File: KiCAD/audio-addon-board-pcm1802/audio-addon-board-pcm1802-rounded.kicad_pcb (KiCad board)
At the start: 4 copper layers, 85 x 70 mm, 69 parts, among them J1 RCA, J2 CONN_HOST_1, J3 RCA, J4 RCA, J5 RCA, SW1 SW_DIP_x04, U1 PCM1802DBR, U2 LTC1682IS8-5, U3 SN74LVC1G125DBV

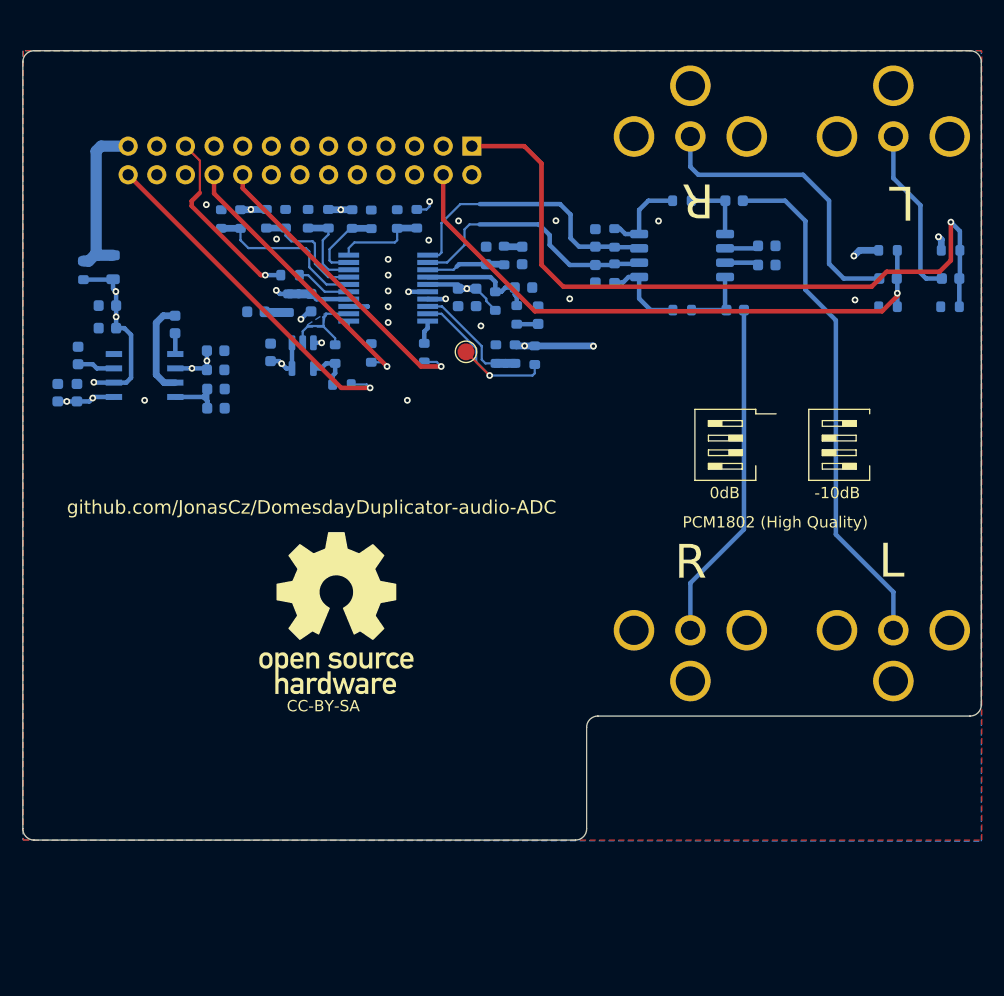
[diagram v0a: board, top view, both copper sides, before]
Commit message: working on layout (2025-10-09 sent to jlc)
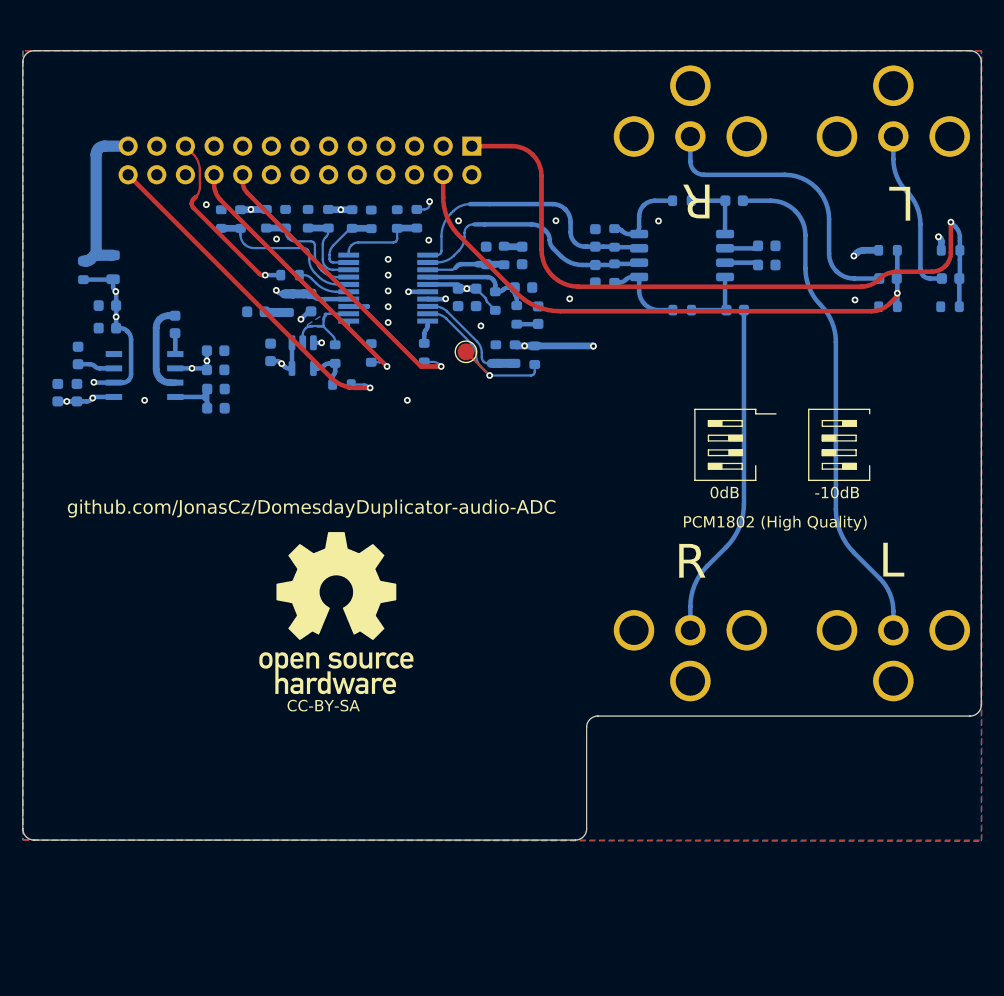
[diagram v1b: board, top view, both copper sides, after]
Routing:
- net +3.3V: track 88.0 -> 86.6 mm
- net /+5V, Analog: track 74.0 -> 72.8 mm
- net Net-(J4-In): track 45.8 -> 44.6 mm
- net Net-(U2-CPO): track 6.17 -> 5.13 mm
- net Net-(J2-Pin_1): track 65.1 -> 64.1 mm
- net Net-(J1-In): track 26.8 -> 26.1 mm
- net GND: track 53.9 -> 53.2 mm
- net Net-(J2-Pin_4): track 53.5 -> 52.8 mm
- net Net-(U1-OSR): track 14.8 -> 14.2 mm
- net VINR: track 23.1 -> 22.5 mm
- net VINL: track 25.0 -> 24.4 mm
- net Net-(J5-In): track 30.4 -> 29.9 mm

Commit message: update board
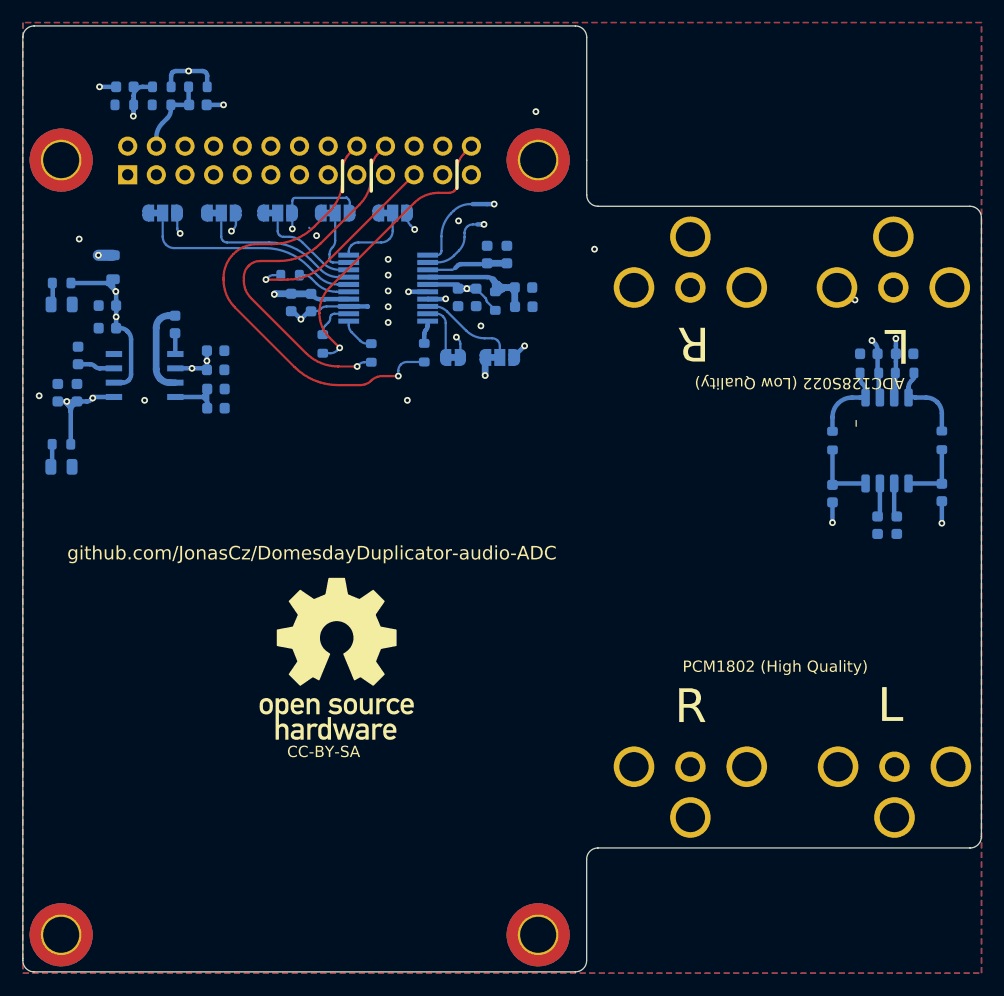
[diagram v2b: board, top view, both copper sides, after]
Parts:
- removed C25: 1uF, Capacitor_SMD:C_0603_1608Metric
- removed R12, RBYPASS1, RFMT0, RFMT1, RMODE0, RMODE1, ROSR1: NP, Resistor_SMD:R_0603_1608Metric
- removed R22: 1R, Resistor_SMD:R_0603_1608Metric
- removed R3, R8, RBYPASS2, RFMT2, RFMT4, RMODE2, RMODE4, ROSR2: 0R, Resistor_SMD:R_0603_1608Metric
- removed TP1: TestPoint, TestPoint:TestPoint_Pad_D1.5mm
- removed U3: SN74LVC1G125DBV, Package_TO_SOT_SMD:SOT-23-5
- added D1: LED, LED_SMD:LED_0805_2012Metric, B.Cu at (103.4, 86.9)
- added D2: LED, LED_SMD:LED_0805_2012Metric, B.Cu at (103.4, 72.5)
- added H1: MountingHole, MountingHole:MountingHole_3.2mm_M3_DIN965_Pad_TopBottom, F.Cu at (103.4, 59.7)
- added H2: MountingHole, MountingHole:MountingHole_3.2mm_M3_DIN965_Pad_TopBottom, F.Cu at (145.7, 59.7)
- added H3: MountingHole, MountingHole:MountingHole_3.2mm_M3_DIN965_Pad_TopBottom, F.Cu at (103.4, 128.4)
- added H4: MountingHole, MountingHole:MountingHole_3.2mm_M3_DIN965_Pad_TopBottom, F.Cu at (145.7, 128.4)
- added JBYPASS1: Jumper, Jumper:SolderJumper-3_P1.3mm_Bridged12_RoundedPad1.0x1.5mm, B.Cu at (142.3, 77.2)
- added JFMT0: Jumper, Jumper:SolderJumper-3_P1.3mm_Bridged12_RoundedPad1.0x1.5mm, B.Cu at (117.6, 64.4)
- added JFMT1: Jumper, Jumper:SolderJumper-3_P1.3mm_Bridged12_RoundedPad1.0x1.5mm, B.Cu at (122.6, 64.4)
- added JFSYNC1: Jumper_2_Small_Bridged, Jumper:SolderJumper-2_P1.3mm_Bridged_RoundedPad1.0x1.5mm, B.Cu at (138.2, 77.2)
- added JMODE0: Jumper, Jumper:SolderJumper-3_P1.3mm_Bridged12_RoundedPad1.0x1.5mm, B.Cu at (132.8, 64.4)
- added JMODE1: Jumper, Jumper:SolderJumper-3_P1.3mm_Bridged12_RoundedPad1.0x1.5mm, B.Cu at (127.7, 64.4)
- added JOSR1: Jumper, Jumper:SolderJumper-3_P1.3mm_Bridged12_RoundedPad1.0x1.5mm, B.Cu at (112.4, 64.4)
- R1, R2: value 1R -> 1k
- moved R11 75.4 mm to (109.0, 54.8)
- moved C23 75.2 mm to (109.0, 53.2)
- moved R14 71.4 mm to (112.3, 53.2), turned to 0 degrees
- moved R9 66.9 mm to (112.3, 54.8)
- moved C24 63.1 mm to (115.5, 54.8), turned to 180 degrees
- moved R13 62.9 mm to (115.5, 53.2), turned to 180 degrees
- moved R1 42.7 mm to (103.4, 84.9), turned to 180 degrees
- moved C12 31.8 mm to (181.5, 89.2), turned to 90 degrees
- moved RA3 31.4 mm to (181.5, 84.5), turned to 90 degrees
- moved J2 30.6 mm to (109.3, 61.0), turned to -90 degrees
- moved C18 29.3 mm to (178.2, 76.9), turned to 180 degrees
- moved RA1 28.4 mm to (178.2, 78.6), turned to 180 degrees
- moved C20 27.3 mm to (177.5, 92.1), turned to -90 degrees
- moved C19 25.3 mm to (175.0, 76.9), turned to 180 degrees
- moved C21 25.1 mm to (175.8, 92.1), turned to -90 degrees
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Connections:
- C15 pad 2: Net-(C15-Pad2) -> +3.3V
- C9 pad 1: Net-(C9-Pad1) -> Net-(U1-VREF1)
- CNP1 pad 1: Net-(CNP1-Pad1) -> Net-(U1-VREF2)
- R1 pad 1: Net-(C9-Pad1) -> /+5V, Analog
- R1 pad 2: Net-(U1-VREF1) -> Net-(D1-A)
- R10 pad 1: Net-(R10-Pad1) -> Net-(U1-DOUT)
- R2 pad 2: Net-(C15-Pad2) -> Net-(D2-A)
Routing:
- net Net-(J3-In): track 14.7 -> 84.3 mm, vias 0 -> 1
- net Net-(J2-Pin_1): track 64.1 -> 13.1 mm
- net Net-(J2-Pin_4): track 52.8 -> 7.05 mm, vias 1 -> 0
- net VINL: track 24.4 -> 56.0 mm, vias 0 -> 2
- net VINR: track 22.5 -> 51.0 mm, vias 0 -> 2
- net Net-(J1-In): track 26.1 -> 51.4 mm, vias 0 -> 2
- net /+3v3 from host: track 15.0 -> 39.9 mm, vias 0 -> 1
- net Net-(J4-In): track 44.6 -> 24.8 mm, vias 0 -> 1
- net GND: track 53.2 -> 69.3 mm, vias 19 -> 16
- net LRCK: track 26.9 -> 41.9 mm
- net +3.3V: track 86.6 -> 73.7 mm, vias 15 -> 14
- net Net-(JFSYNC1-B): track 16.1 -> 5.12 mm, vias 1 -> 0
- net BCK: track 24.8 -> 33.9 mm
- net /+5V, Analog: track 72.8 -> 77.9 mm
- net Net-(JOSR1-C): track 14.2 -> 19.3 mm
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- removed copper zone on B.Cu, net Net-(U1-DOUT)
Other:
- board size 85 x 70 mm -> 85 x 83.9 mm
- board text added: "*"
- board text added: "3v3"
- board text added: "5V"
- board text added: "ADC128S022 (Low Quality)"
- board text added: "JLCJLCJLCJLC"
- board text removed: "JLCJLCJLC"
